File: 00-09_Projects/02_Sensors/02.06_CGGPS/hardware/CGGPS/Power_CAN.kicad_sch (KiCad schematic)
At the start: 22 parts, among them J1 USB_C_Receptacle_USB2.0_14P, J4 Conn_01x04_Socket, U4 SN65HVD230, U5 AP2210K-3.3TRG1

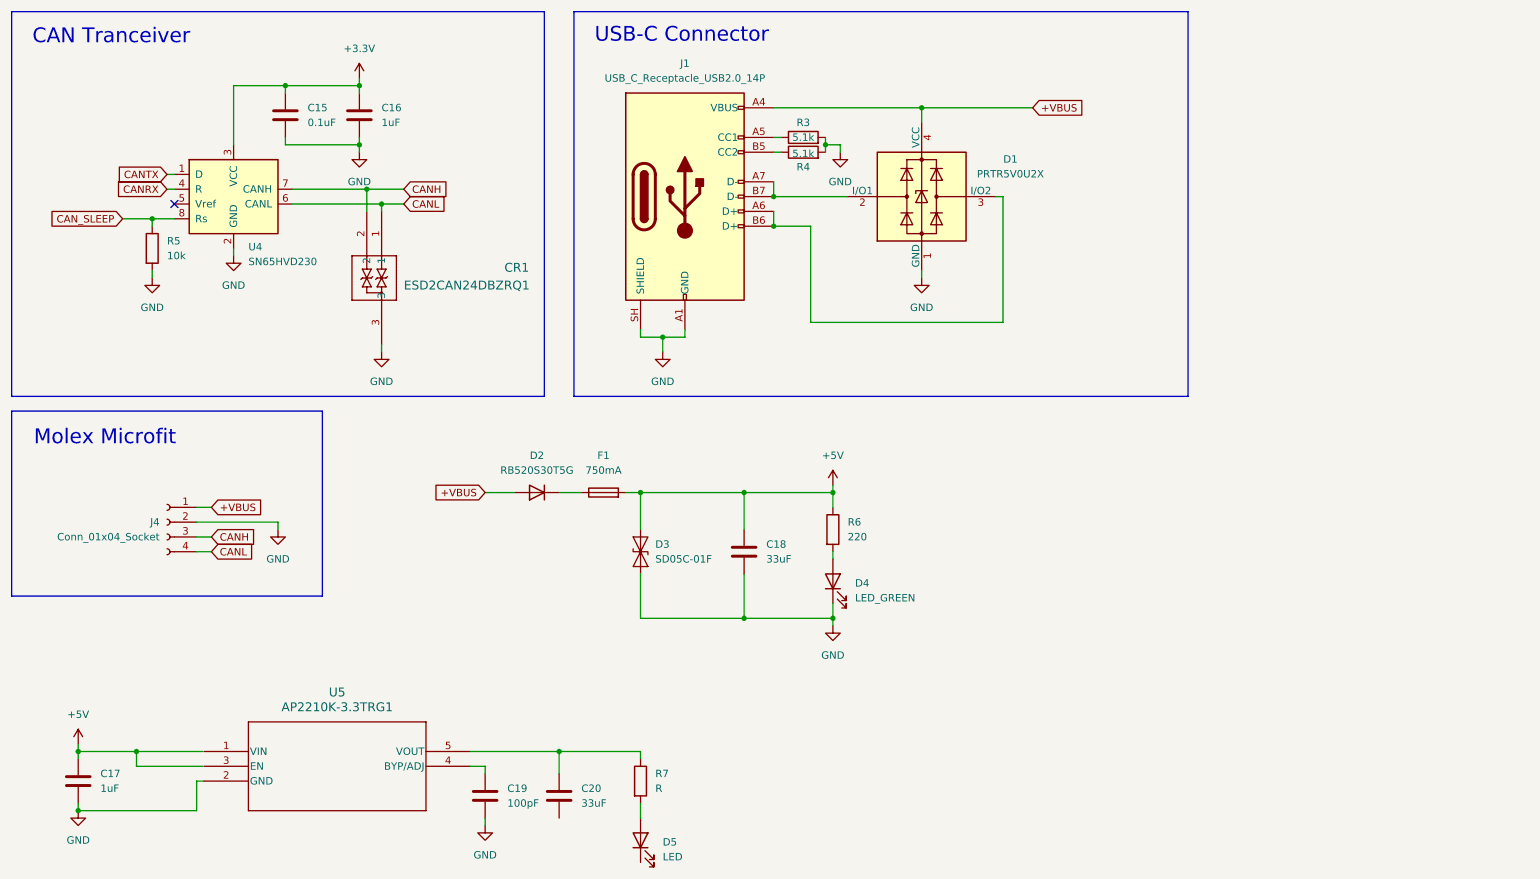
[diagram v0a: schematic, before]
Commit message: wip
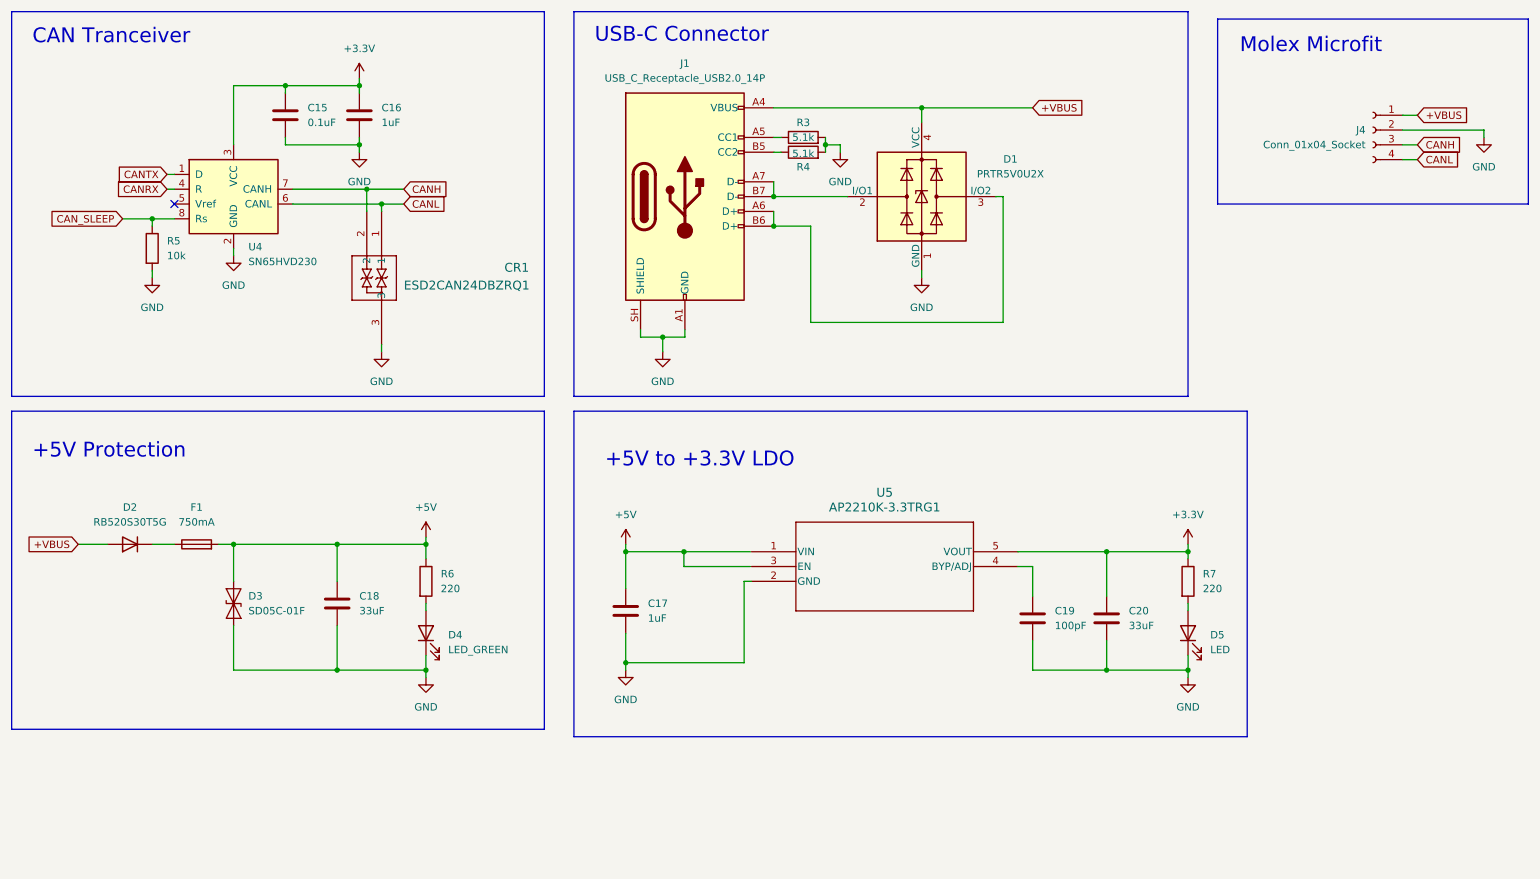
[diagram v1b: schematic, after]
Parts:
- R7: value R -> 220
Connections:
- net +3.3V: now also C20.1, R7.1, U5.5 (VOUT)
- net GND: now also C20.2, D5.1 (K)
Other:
- note added: "+5V Protection"
- note added: "+5V to +3.3V LDO"
- moved on the sheet: C17, C18, C19, C20, D2, D3, D4, D5, F1, J4, R6, R7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
